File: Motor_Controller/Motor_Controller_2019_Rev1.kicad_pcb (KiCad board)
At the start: 2 copper layers, 124.4 x 86.1 mm, 242 parts, among them Q12 Q_NMOS_DGS, Q13 Q_NMOS_DGS, Q14 Q_NMOS_DGS, Q15 Q_NMOS_DGS, Q16 Q_NMOS_DGS, Q17 Q_NMOS_DGS, Q4 Q_NMOS_DGS, Q5 Q_NMOS_DGS, Q6 Q_NMOS_DGS, Q7 Q_NMOS_DGS, Q8 Q_NMOS_DGS, Q9 Q_NMOS_DGS, U1 DCA56_6P35X3P61, U2 NUP4201MR6, U3 LAUNCHXL_F28069M_Launchpad, U4 MAX_3232, U5 DRV8301, U6 NUP4201MR6

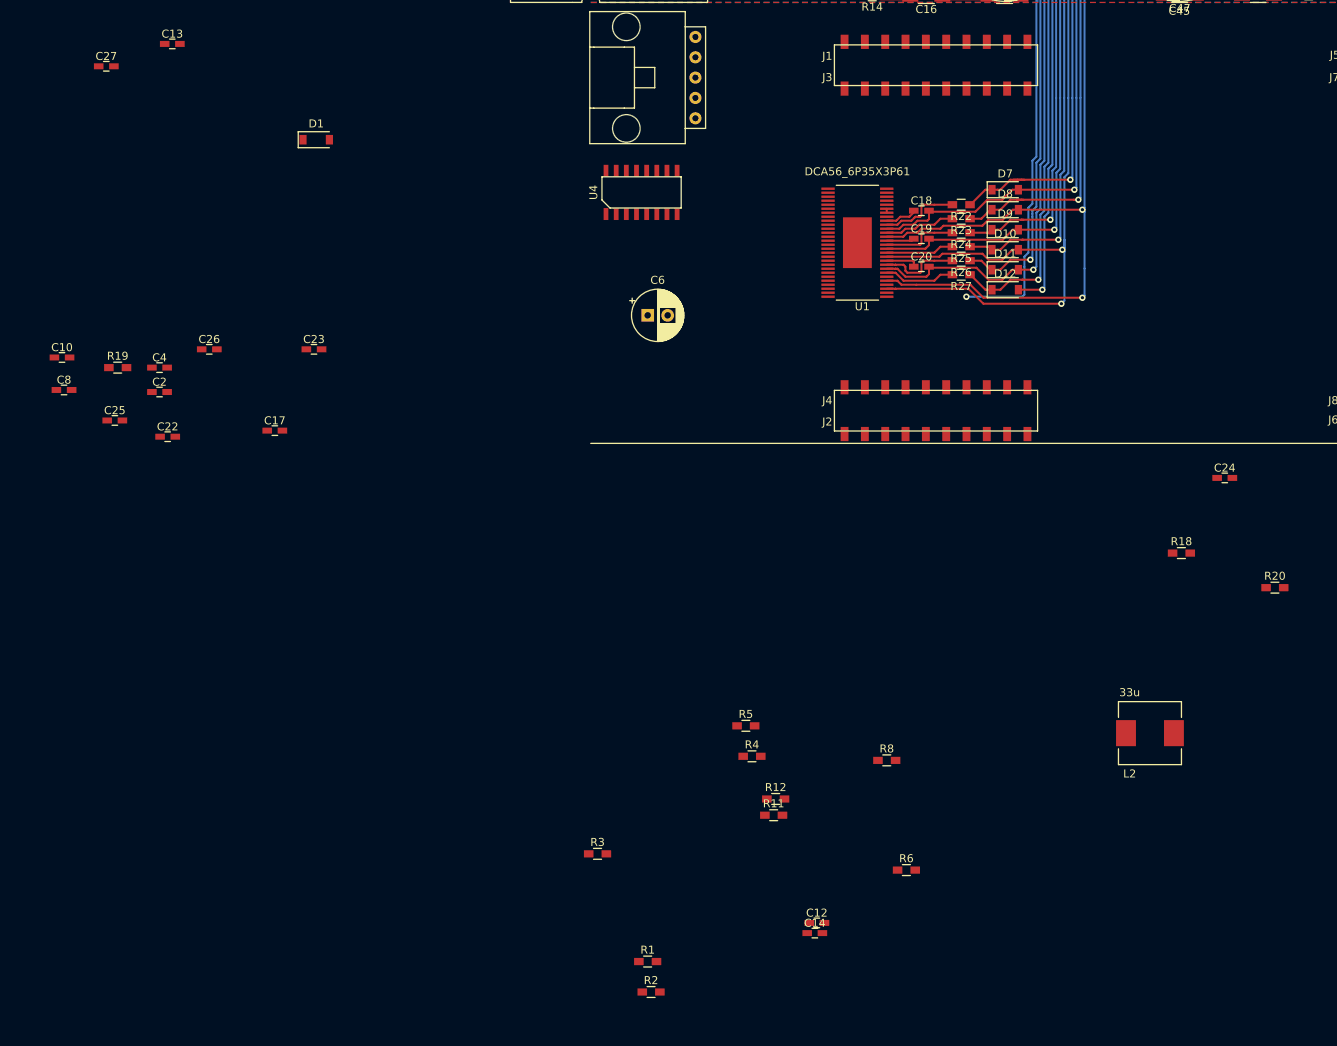
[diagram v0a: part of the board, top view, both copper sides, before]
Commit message: Began work on signal traces
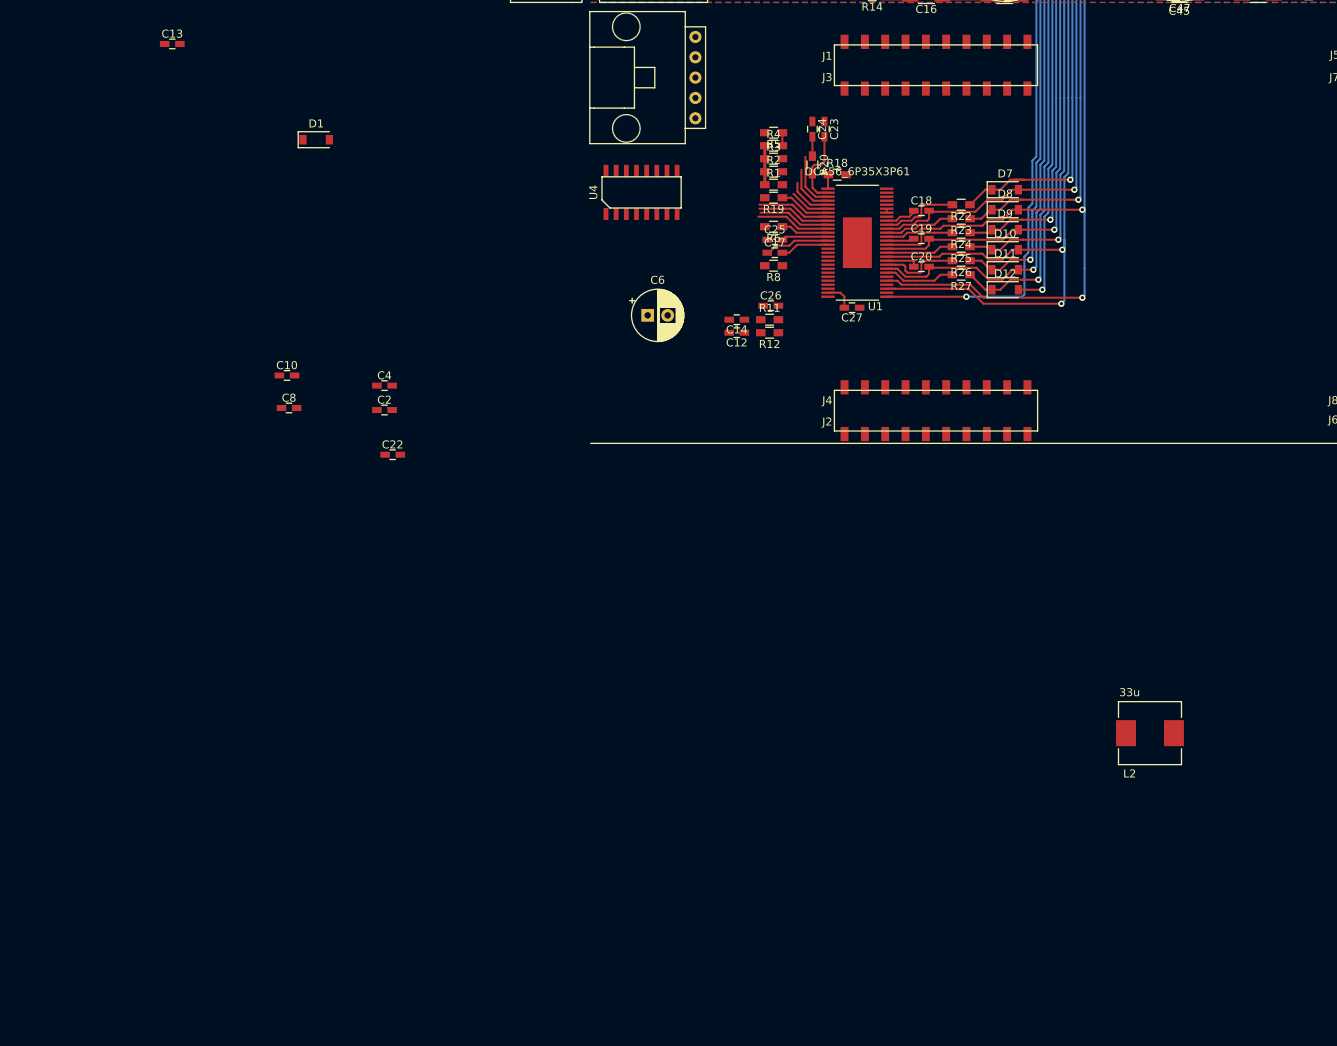
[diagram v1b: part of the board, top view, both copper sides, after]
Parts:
- moved R2 103.7 mm to (73.4, 50.6)
- moved R1 98.4 mm to (73.4, 52.2)
- moved C27 98.0 mm to (83.2, 67.6), turned to 180 degrees
- moved R3 89.6 mm to (73.4, 49.0)
- moved C25 85.5 mm to (73.5, 59.1)
- moved R19 84.7 mm to (73.4, 53.9), turned to 180 degrees
- moved R6 82.1 mm to (73.4, 57.5), turned to 180 degrees
- moved R20 78.3 mm to (78.2, 49.8), turned to 270 degrees
- moved C14 77.3 mm to (68.8, 69.1), turned to 180 degrees
- moved R4 76.4 mm to (73.4, 47.4)
- moved C12 74.5 mm to (68.8, 70.8), turned to 180 degrees
- moved R5 74.2 mm to (73.4, 45.8), turned to 180 degrees
- moved C26 70.4 mm to (73.0, 67.4)
- moved C23 69.5 mm to (79.8, 45.3), turned to 270 degrees
- moved C24 67.5 mm to (78.2, 45.3), turned to 270 degrees
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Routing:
- net PVDD_M1: track 67.2 -> 77.2 mm
- net Net-(C23-Pad2): track 0.00 -> 9.71 mm
- net SCLK_M1: track 0.00 -> 9.33 mm
- net SDI_M1: track 0.00 -> 9.20 mm
- net NSCS_M1: track 0.00 -> 9.20 mm
- net SDO_M1: track 0.00 -> 9.08 mm
- net Net-(R4-Pad2): track 0.00 -> 8.72 mm
- net Net-(C17-Pad1): track 0.00 -> 8.23 mm
- net Net-(R19-Pad1): track 0.00 -> 6.63 mm
- net PWRGD_M1: track 0.00 -> 6.33 mm
- net Net-(C17-Pad2): track 0.00 -> 6.12 mm
- net DC_CAL_M1: track 0.00 -> 6.02 mm
- net Net-(C25-Pad2): track 0.00 -> 5.86 mm
- net NOCTW_M1: track 0.00 -> 5.63 mm
- net NFAULT_M1: track 0.00 -> 5.36 mm
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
